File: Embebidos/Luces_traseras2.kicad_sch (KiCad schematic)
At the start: 12 parts, among them IC2 DMP3056LSD-13, J8 RJ45, J9 RJ45

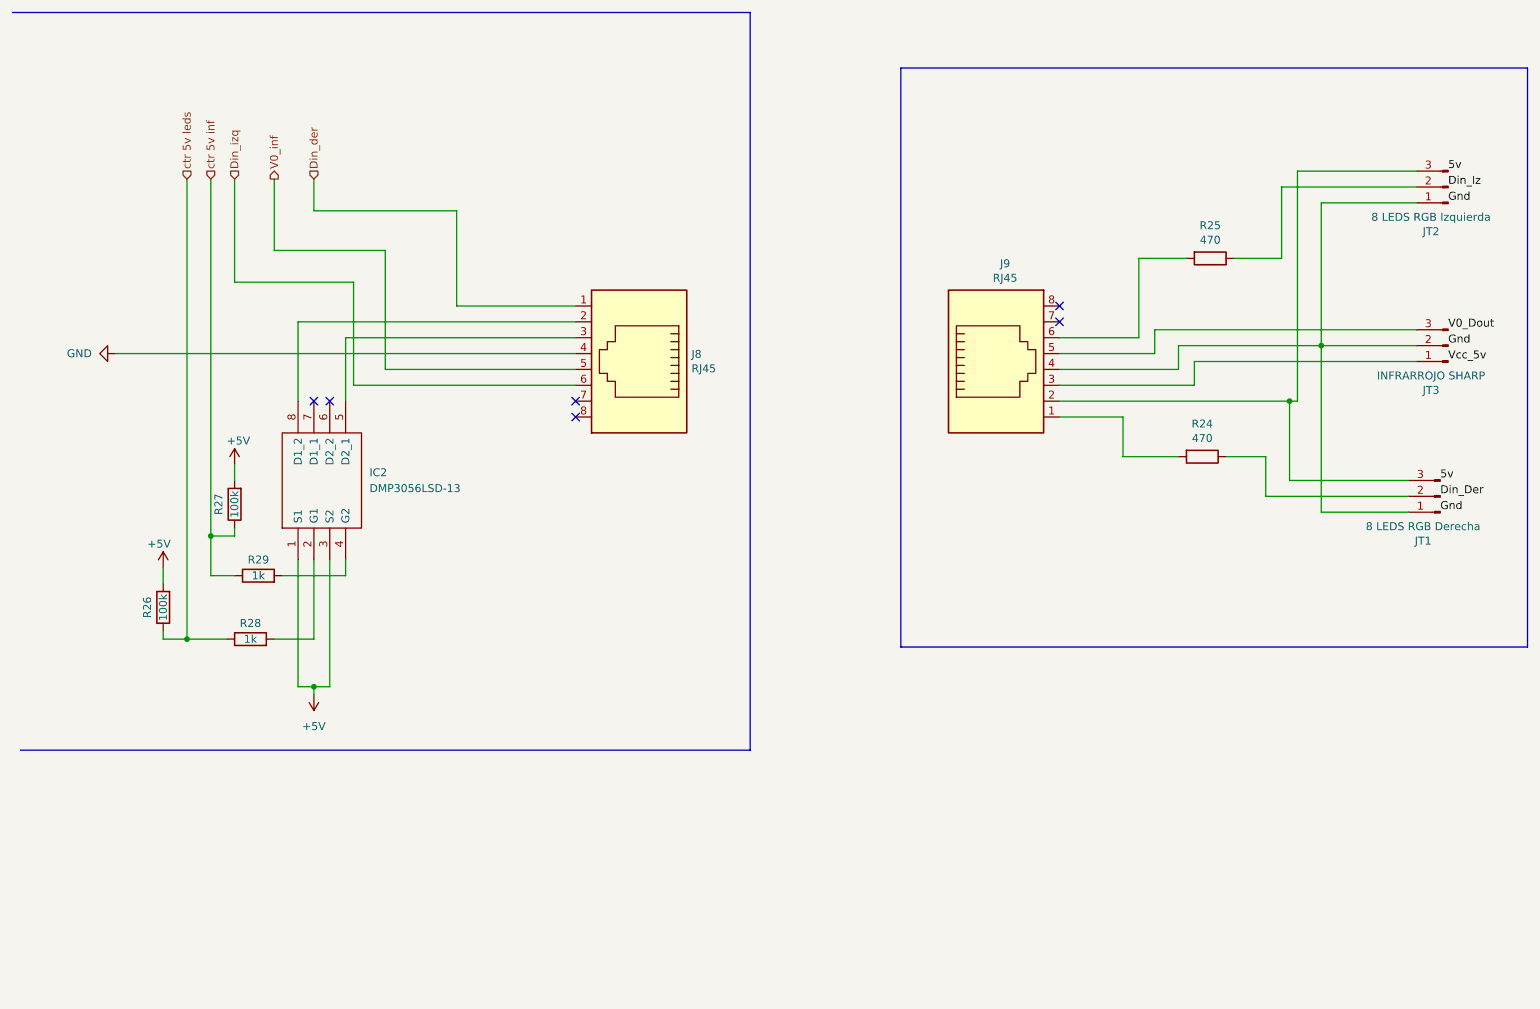
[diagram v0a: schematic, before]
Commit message: transistores traseros
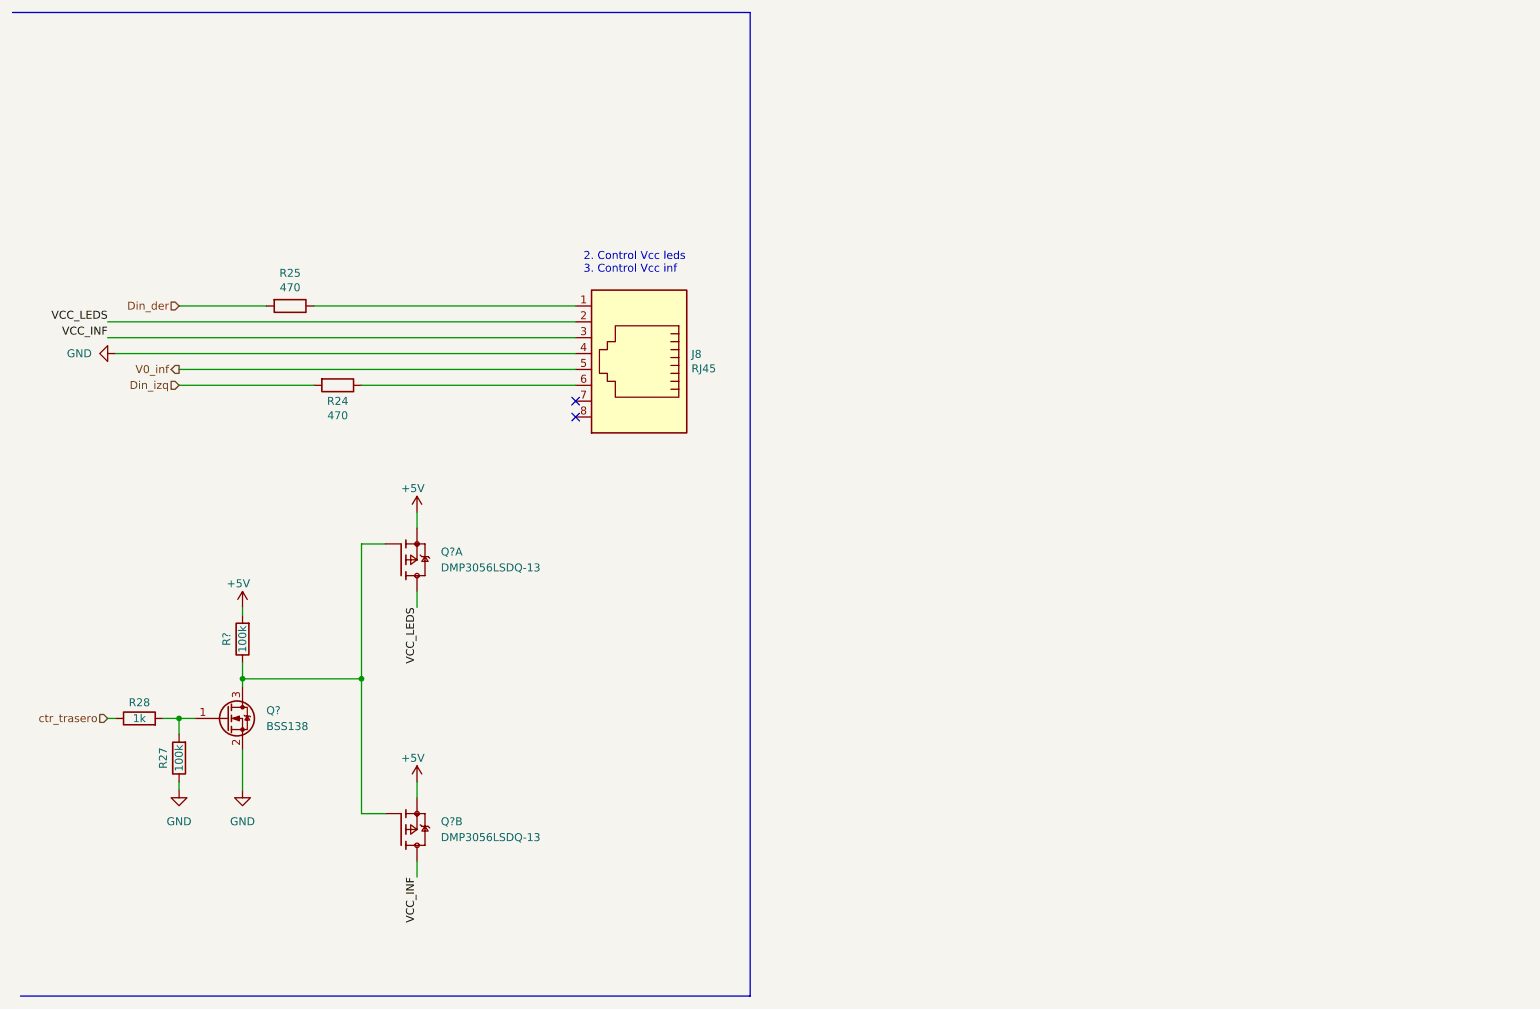
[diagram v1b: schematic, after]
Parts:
- removed IC2: DMP3056LSD-13, SOIC127P600X175-8N, symbol DMP3056LSD-13:DMP3056LSD-13
- removed J9: RJ45, symbol Connector:RJ45
- removed JT1: 8 LEDS RGB Derecha, symbol Connector:Conn_01x03_Male
- removed JT2: 8 LEDS RGB Izquierda, symbol Connector:Conn_01x03_Male
- removed JT3: INFRARROJO SHARP, symbol Connector:Conn_01x03_Male
- removed R26: 100k, symbol Device:R
- removed R29: 1k, symbol Device:R
- added Q?: BSS138, Package_TO_SOT_SMD:SOT-23, symbol Transistor_FET:BSS138
- added Q? (x2): DMP3056LSDQ-13, DMP3056LSD:SOIC127P600X175-8N, symbol DMP3056LSDQ-13:DMP3056LSDQ-13
- added R?: 100k, symbol Device:R
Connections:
- net ctr 5v inf is gone; now on net GND: R27.1
- net +5V: now also Q?.1, Q?.3, R?.2; no longer R27.2
- net Din_der: now also R25.2; no longer J8.1
- net Din_izq: now also R24.2; no longer J8.6
- net GND: now also Q?.2 (S)
- net at R25.1: now also J8.1
- net at R24.1: now also J8.6
- net VCC_LEDS: now reaches J8.2
- net VCC_LEDS: now also Q?.7, Q?.8
- net VCC_INF: now reaches J8.3
- net VCC_INF: now also Q?.5, Q?.6
- net at R28.2: now also R27.2, Q?.1 (G)
- net ctr 5v leds renamed ctr_trasero
- new net: Q?.2, Q?.3 (D), Q?.4, R?.1
- no-connect marks 6 -> 2
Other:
- note added: "2. Control Vcc leds 3. Control Vcc inf"
- moved on the sheet: R24, R25, R27, R28
